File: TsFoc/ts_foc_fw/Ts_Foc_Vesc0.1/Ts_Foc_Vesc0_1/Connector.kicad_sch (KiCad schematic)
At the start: 20 parts, among them CN1 MR30PW-M30.G.Y, CN10 GH1.25-4P, CN11 GH1.25-5PLT, CN12 GH1.25-5PLT, CN13 GH1.25-4P, CN2 MR30PW-M30.G.Y, CN3 GH1.25-2P_LT, CN4 GH1.25-2P_LT, CN5 XT30PW-M, CN6 GH1.25-4P, CN7 GH1.25-4P, CN8 GH1.25-4P, CN9 GH1.25-4P

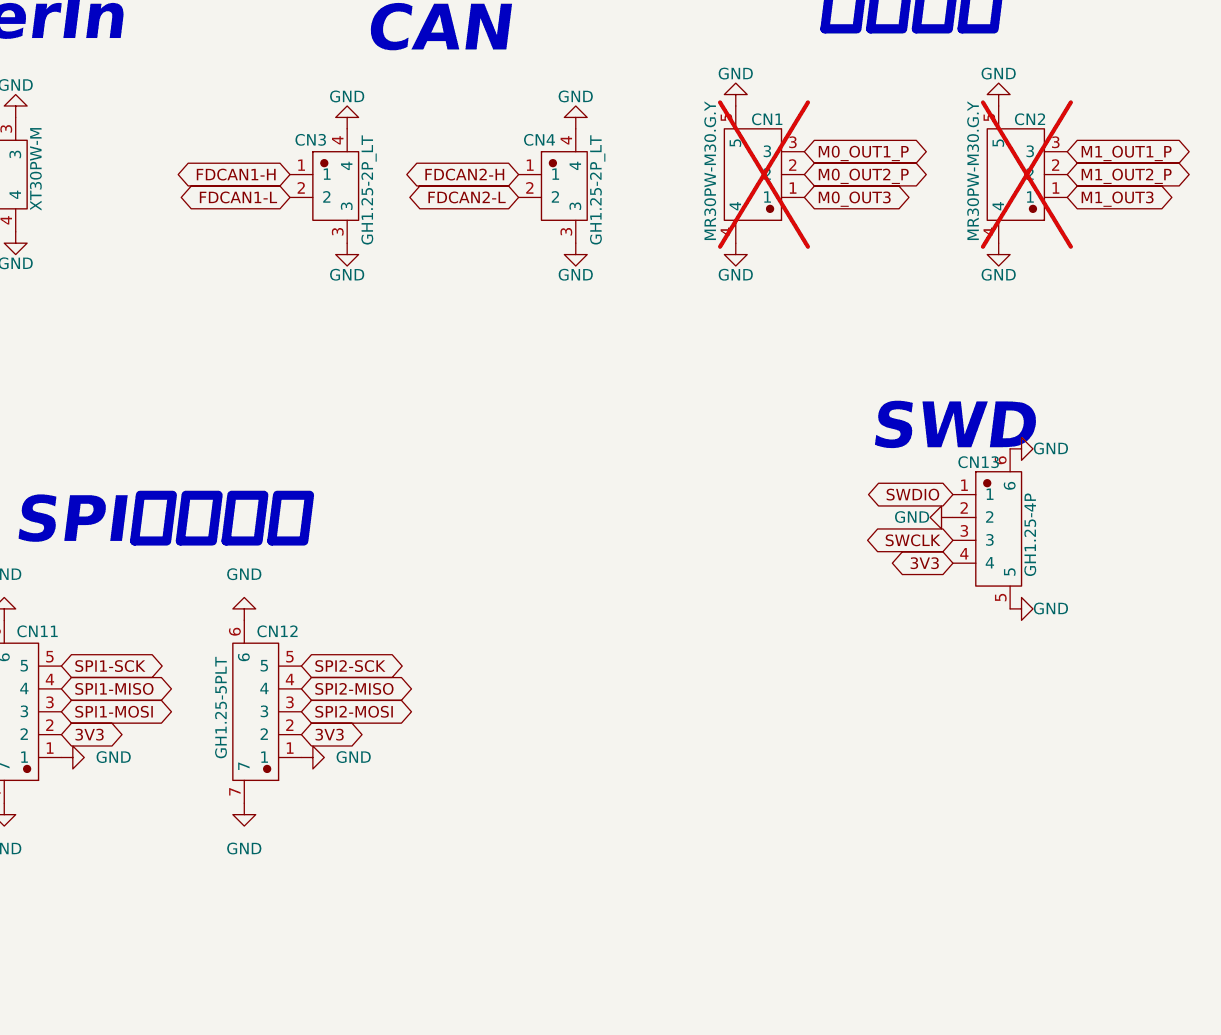
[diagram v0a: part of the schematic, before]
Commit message: 第一版layout完成，准备打板验证
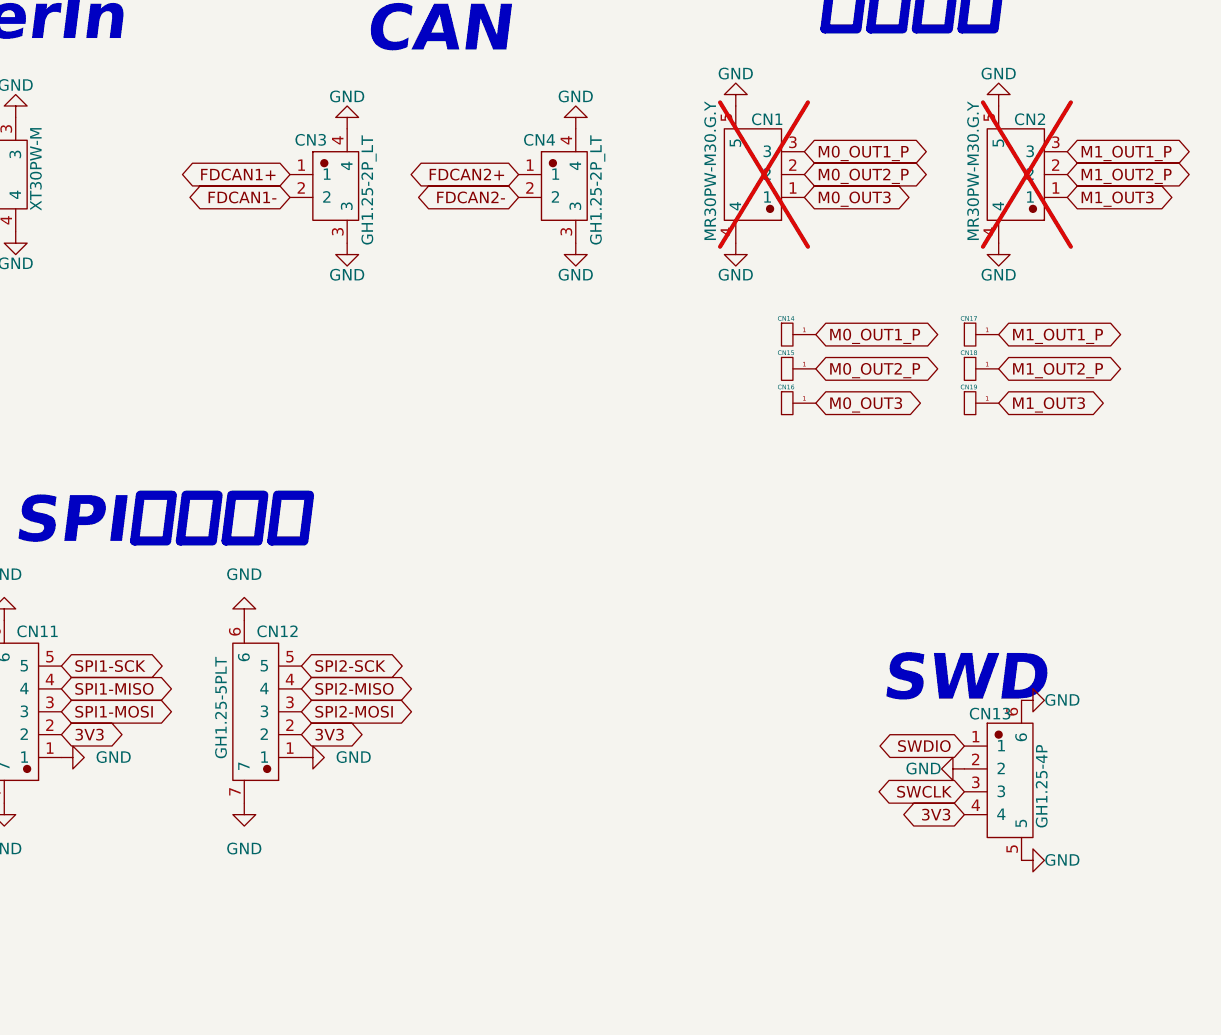
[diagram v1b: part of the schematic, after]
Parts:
- added CN14, CN15, CN16, CN17, CN18, CN19: ~, Ts_Foc_Vo封装库:通孔焊盘, symbol Ts_Foc_Vo符号库:通孔焊盘
- CN1, CN2: footprint Ts_Foc_Vo封装库:MR30PW-M30-G-Y -> (none)
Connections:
- net M0_OUT1_P: now also CN14.1
- net M0_OUT2_P: now also CN15.1
- net M0_OUT3: now also CN16.1
- net M1_OUT1_P: now also CN17.1
- net M1_OUT2_P: now also CN18.1
- net M1_OUT3: now also CN19.1
- net FDCAN1-H renamed FDCAN1+
- net FDCAN1-L renamed FDCAN1-
- net FDCAN2-H renamed FDCAN2+
- net FDCAN2-L renamed FDCAN2-
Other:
- moved on the sheet: CN13

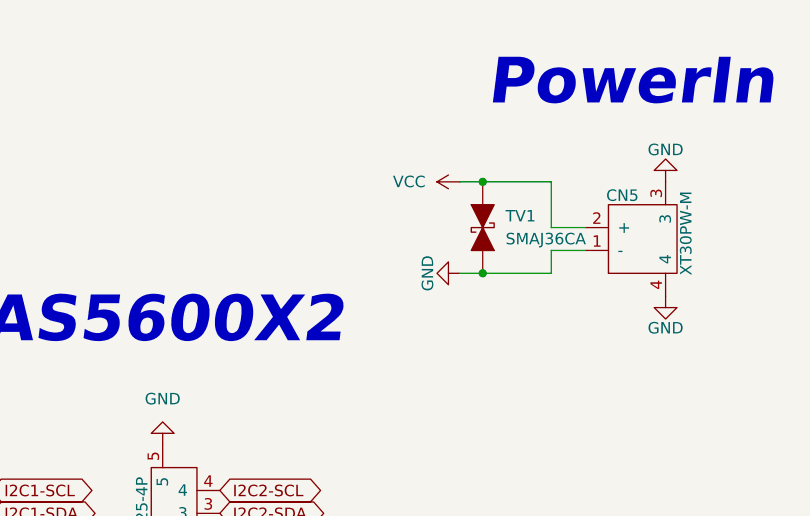
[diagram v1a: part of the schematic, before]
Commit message: 同步_Tue Feb  4 22:38:42     2025
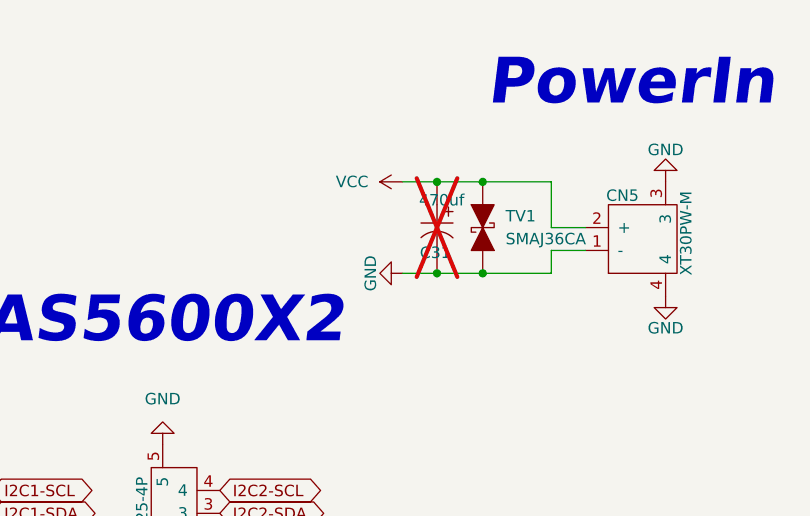
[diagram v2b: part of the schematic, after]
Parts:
- added C31: 470uf, Ts_Foc_Vo封装库:Cap_Electrolytic, symbol Ts_Foc_Vo符号库:Cap_Electrolytic
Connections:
- net GND: now also C31.2
- net VCC: now also C31.1
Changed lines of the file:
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@@
 	)
 	(junction
+		(at 124.46 33.02)
+		(diameter 0)
+		(color 0 0 0 0)
+	)
+	(junction
+		(at 124.46 43.18)
+		(diameter 0)
+		(color 0 0 0 0)
+	)
+	(junction
 		(at 129.54 43.18)
 		(diameter 0)
@@
 	(wire
 		(pts
-			(xy 127 33.02) (xy 129.54 33.02)
+			(xy 120.65 33.02) (xy 124.46 33.02)
 		)
 		(stroke
@@
 	(wire
 		(pts
-			(xy 127 43.18) (xy 129.54 43.18)
+			(xy 120.65 43.18) (xy 124.46 43.18)
 		)
 		(stroke
@@
 	(wire
 		(pts
+			(xy 124.46 43.18) (xy 129.54 43.18)
+		)
+		(stroke
+			(width 0)
+			(type default)
+		)
+	)
+	(wire
+		(pts
+			(xy 124.46 33.02) (xy 129.54 33.02)
+		)
+		(stroke
+			(width 0)
+			(type default)
+		)
+	)
+	(wire
+		(pts
 			(xy 129.54 33.02) (xy 137.16 33.02)
 		)
@@
 	(symbol
 		(lib_id "power:GND")
-		(at 127 43.18 270)
+		(at 120.65 43.18 270)
 		(unit 1)
 		(exclude_from_sim no)
@@
 		(dnp no)
 		(property "Reference" "#PWR057"
-			(at 120.65 43.18 0)
+			(at 114.3 43.18 0)
 			(effects
 				(font
@@
 		)
 		(property "Value" "GND"
-			(at 123.444 43.18 0)
+			(at 117.094 43.18 0)
 			(effects
 				(font
@@
 		)
 		(property "Footprint" ""
-			(at 127 43.18 0)
+			(at 120.65 43.18 0)
 			(effects
 				(font
@@
 		)
 		(property "Datasheet" ""
-			(at 127 43.18 0)
+			(at 120.65 43.18 0)
 			(effects
 				(font
@@
 		)
 		(property "Description" "Power symbol creates a global label with name \"GND\" , ground"
-			(at 127 43.18 0)
+			(at 120.65 43.18 0)
 			(effects
 				(font
@@
 	(symbol
 		(lib_id "power:VCC")
-		(at 127 33.02 90)
+		(at 120.65 33.02 90)
 		(unit 1)
 		(exclude_from_sim no)
@@
 		(fields_autoplaced yes)
 		(property "Reference" "#PWR056"
-			(at 130.81 33.02 0)
+			(at 124.46 33.02 0)
 			(effects
 				(font
@@
 		)
 		(property "Value" "VCC"
-			(at 123.19 33.0199 90)
+			(at 116.84 33.0199 90)
 			(effects
 				(font
@@
 		)
 		(property "Footprint" ""
-			(at 127 33.02 0)
+			(at 120.65 33.02 0)
 			(effects
 				(font
@@
 		)
 		(property "Datasheet" ""
-			(at 127 33.02 0)
+			(at 120.65 33.02 0)
 			(effects
 				(font
@@
 		)
 		(property "Description" "Power symbol creates a global label with name \"VCC\""
-			(at 127 33.02 0)
+			(at 120.65 33.02 0)
 			(effects
 				(font
@@
 					(unit 1)
 				)
+			)
+		)
+	)
+	(symbol
+		(lib_id "Ts_Foc_Vo符号库:Cap_Electrolytic")
+		(at 124.46 38.1 270)
+		(unit 1)
+		(exclude_from_sim yes)
+		(in_bom no)
+		(on_board no)
+		(dnp yes)
+		(property "Reference" "C31"
+			(at 125.984 40.894 90)
+			(effects
+				(font
+					(size 1.27 1.27)
+				)
+				(justify right)
+			)
+		)
+		(property "Value" "470uf"
+			(at 127.508 35.052 90)
+			(effects
+				(font
+					(size 1.27 1.27)
+				)
+				(justify right)
+			)
+		)
+		(property "Footprint" "Ts_Foc_Vo封装库:Cap_Electrolytic"
+			(at 121.666 38.354 0)
+			(effects
+				(font
+					(size 1.27 1.27)
+				)
+				(hide yes)
+			)
+		)
+		(property "Datasheet" ""
+			(at 118.618 38.1 0)
+			(effects
+				(font
+					(size 1.27 1.27)
+				)
+				(hide yes)
+			)
+		)
+		(property "Description" ""
+			(at 124.46 38.1 0)
+			(effects
+				(font
+					(size 1.27 1.27)
+				)
+				(hide yes)
+			)
+		)
+		(property "SuppliersPartNumber" "C2960233"
+			(at 121.666 37.846 0)
+			(effects
+				(font
+					(size 1.27 1.27)
+				)
+				(hide yes)
+			)
+		)
+		(property "uuid" "std:f2c4c4acb06341a6b501ff67d9191846"
+			(at 121.666 37.846 0)
+			(effects
+				(font
+					(size 1.27 1.27)
+				)
+				(hide yes)
+			)
+		)
+		(pin "2"
+		)
+		(pin "1"
+		)
+		(instances
+			(project "Ts_Foc_Vo1_0"
+				(path "/0cbcabec-8024-48c7-ab91-86e279a5637e/f3329442-eac4-40be-b987-eebdbe922017"
+					(reference "C31")
+					(unit 1)
+				)
